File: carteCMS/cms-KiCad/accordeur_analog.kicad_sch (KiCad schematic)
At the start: 18 parts, among them U1 LM358, U2 max7426cua+T, U4 CD4093BM96

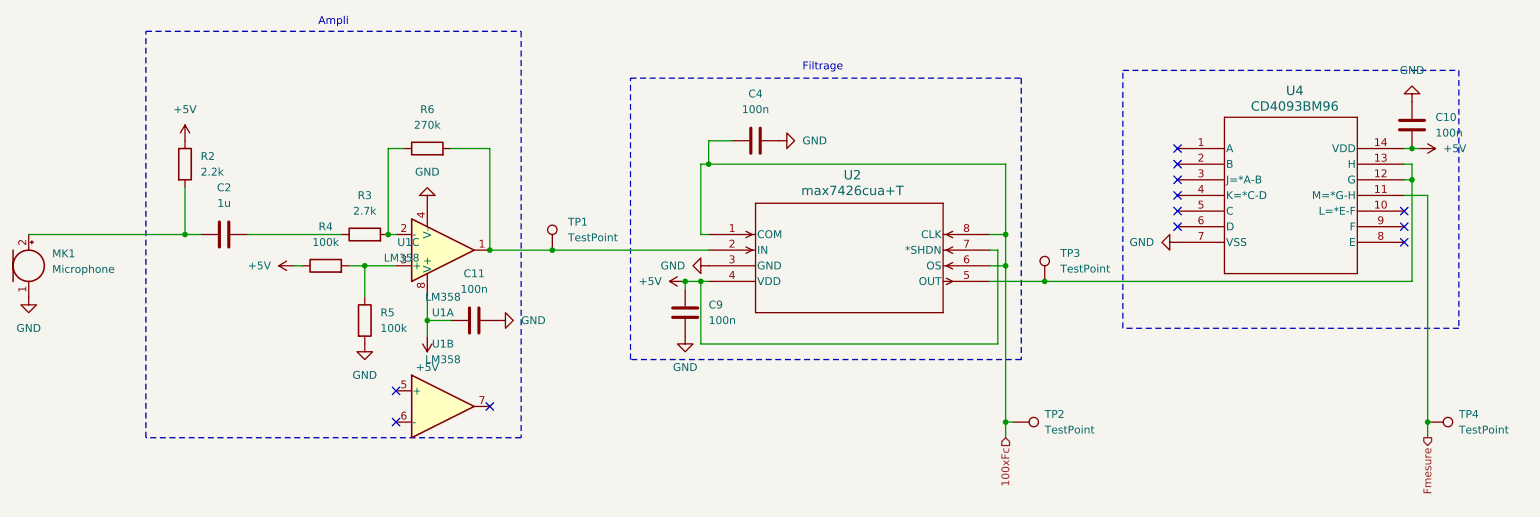
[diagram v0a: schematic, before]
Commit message: v2 - schéma et empruntes terminés (normalement)
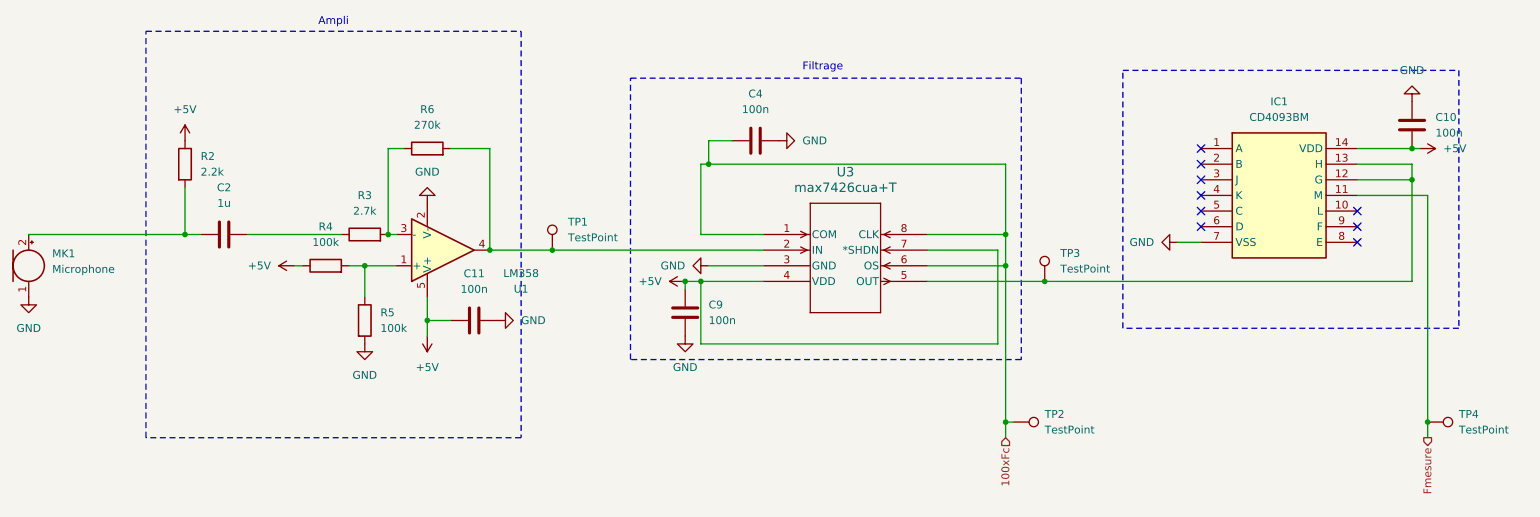
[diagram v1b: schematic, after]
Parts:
- removed U1: LM358, accordeurEmp:LM358emp, symbol Amplifier_Operational:LM358
- removed U2: max7426cua+T, 21-0036K_MXM, symbol 2026-09-04_07-21-49:max7426cua+T
- removed U4: CD4093BM96, D14, symbol 2026-09-04_07-53-46:CD4093BM96
- added IC1: CD4093BM, Package_SO:SO-14_5.3x10.2mm_P1.27mm, symbol accordeurSym:CD4093BM
- added U1: LM358, Package_TO_SOT_SMD:SOT-353_SC-70-5, symbol Amplifier_Operational:TLV172IDCK
- added U3: max7426cua+T, accordeurEmp:MAX7426, symbol accordeurSym:max7426cua+T
- C10, C11, C9: footprint (none) -> Capacitor_SMD:C_0805_2012Metric
- MK1: footprint (none) -> accordeurEmp:micro-KECG2740PBJ
- TP1, TP2, TP3, TP4: footprint (none) -> TestPoint:TestPoint_Pad_D2.0mm
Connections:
- net +5V: now also IC1.14 (VDD), U1.5 (V+), U3.4 (VDD), U3.7 (*SHDN)
- net 100xFc: now also U3.1 (COM), U3.6 (OS), U3.8 (CLK)
- net Fmesure: now also IC1.11 (M)
- net GND: now also IC1.7 (VSS), U1.2 (V-), U3.3 (GND)
- net at R6.2, TP1.1: now also U1.4, U3.2 (IN)
- net at TP3.1: now also IC1.12 (G), IC1.13 (H), U3.5 (OUT)
- net at R4.2, R5.1: now also U1.1 (+)
- net at R3.2, R6.1: now also U1.3 (-)
- no-connect marks 12 -> 9
